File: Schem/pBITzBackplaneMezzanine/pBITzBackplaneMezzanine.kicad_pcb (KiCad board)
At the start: 4 copper layers, 139 x 130 mm, 52 parts, among them J1 USB3_A_Stacked, J2 Conn_01x04, J3 Conn_01x04, J4 10067847-001RLF, J5 FH69-60S-0.5SH, J6 pBITzBus, J7 FH69-60S-0.5SH, SW1 SW_Coded_SH-7030, SW2 SW_Coded_SH-7030, U1 FE1.1S-BSOP28BCN, U2 MAX3421EETJ_T, U3 CD74HC4050M96, U4 CD74HC4050M96, U5 74HC688, U6 74HC688, Y1 ABL-12.000MHZ-B2, Y2 ABL-12.000MHZ-B2

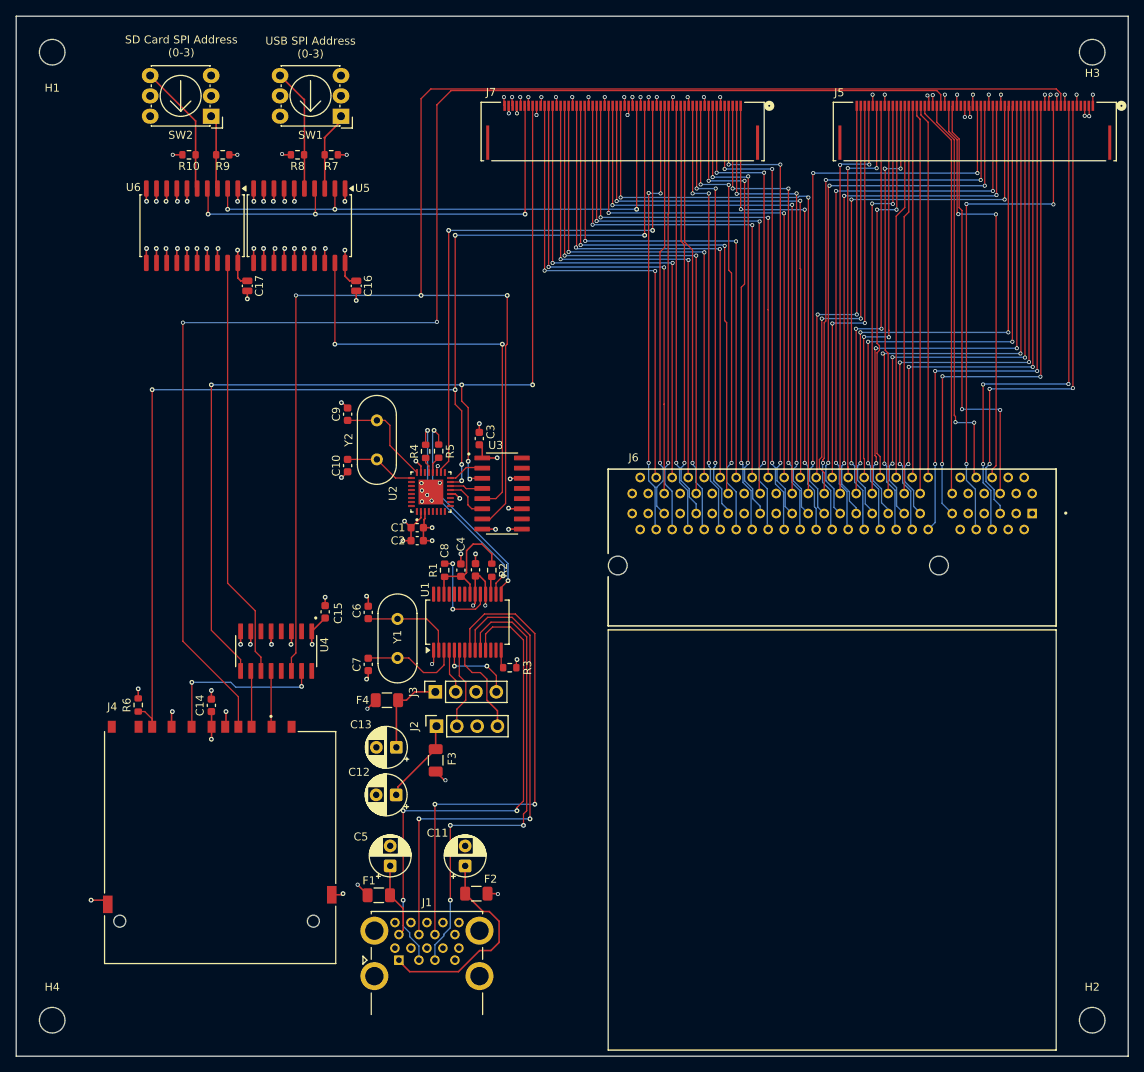
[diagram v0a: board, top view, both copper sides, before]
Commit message: synching
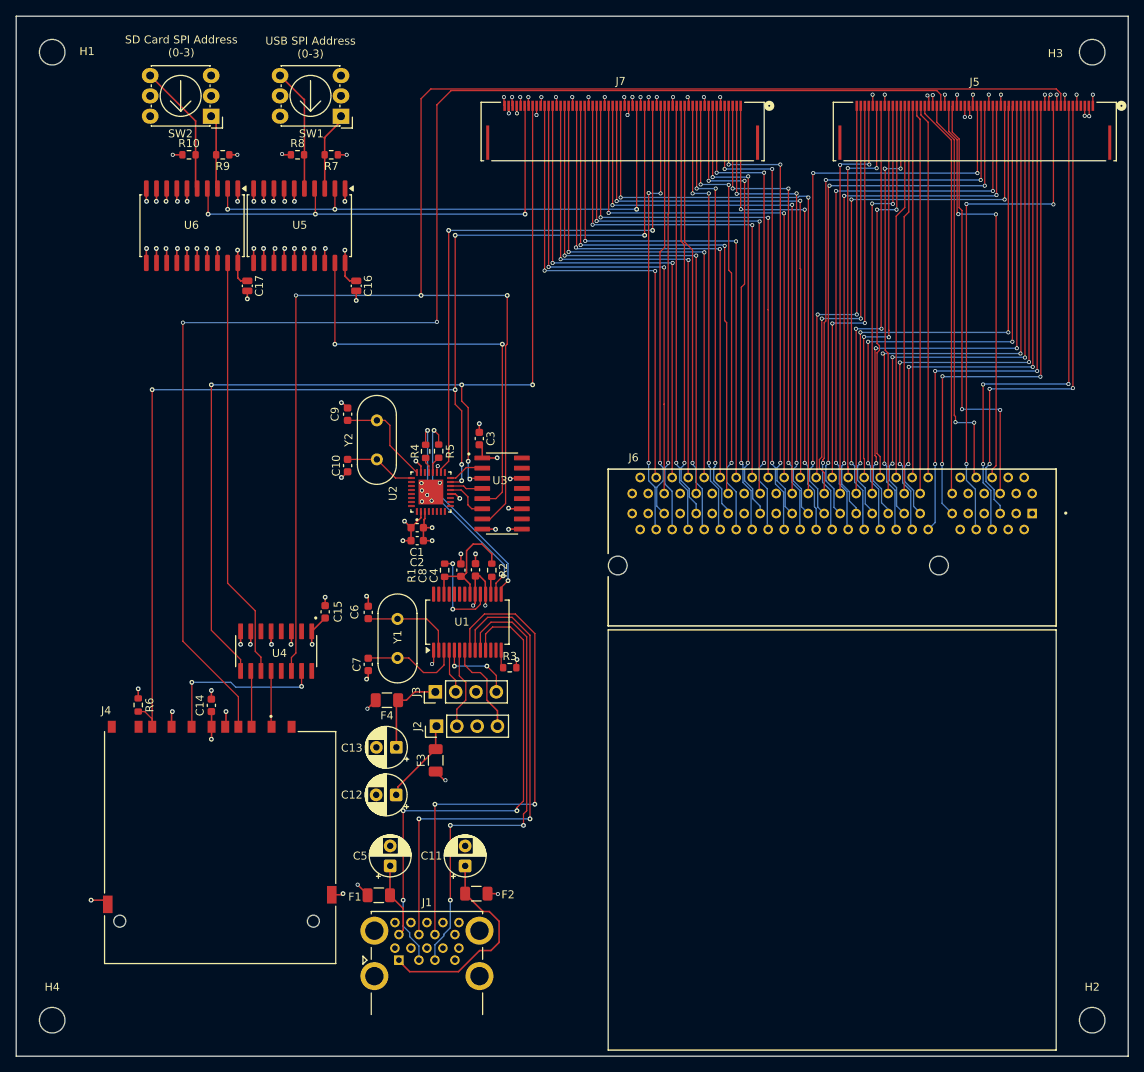
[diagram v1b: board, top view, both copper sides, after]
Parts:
- J2, J3: footprint Connector_PinSocket_2.54mm:PinSocket_1x04_P2.54mm_Vertical -> Connector_PinHeader_2.54mm:PinHeader_1x04_P2.54mm_Vertical
